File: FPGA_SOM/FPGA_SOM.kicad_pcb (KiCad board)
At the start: 6 copper layers, 42 x 38 mm, 47 parts, among them J102 Conn_01x14, J103 Conn_01x09, J104 Conn_01x11, J105 Conn_01x02, J106 Conn_01x06, U102 AP2127N-3.3, U103 W25X20CLSN, U104 AP2127N-1.2, U105 ICE40UP5K-SG48ITR, X101 ECS-2520MV-xxx-xx

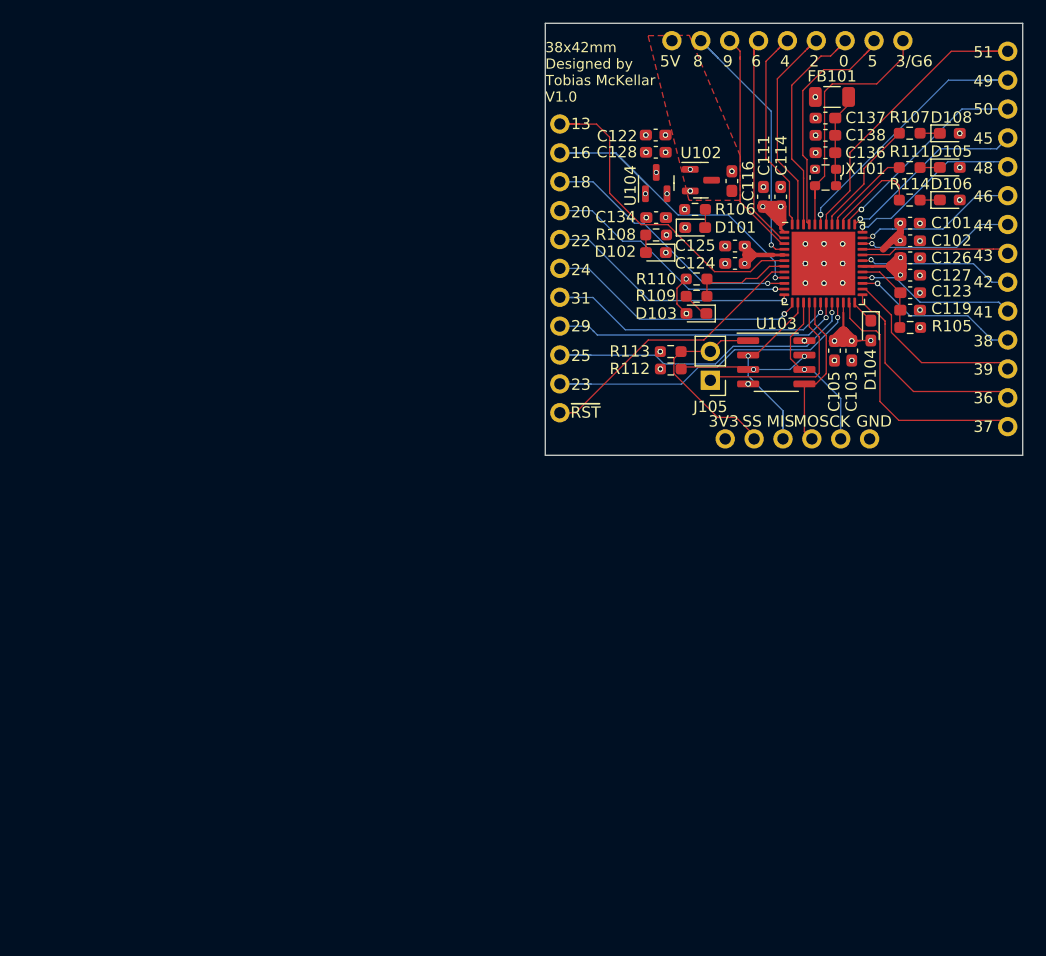
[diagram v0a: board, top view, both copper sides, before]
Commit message: First attempt at V2. Likely to be changed in the near future.
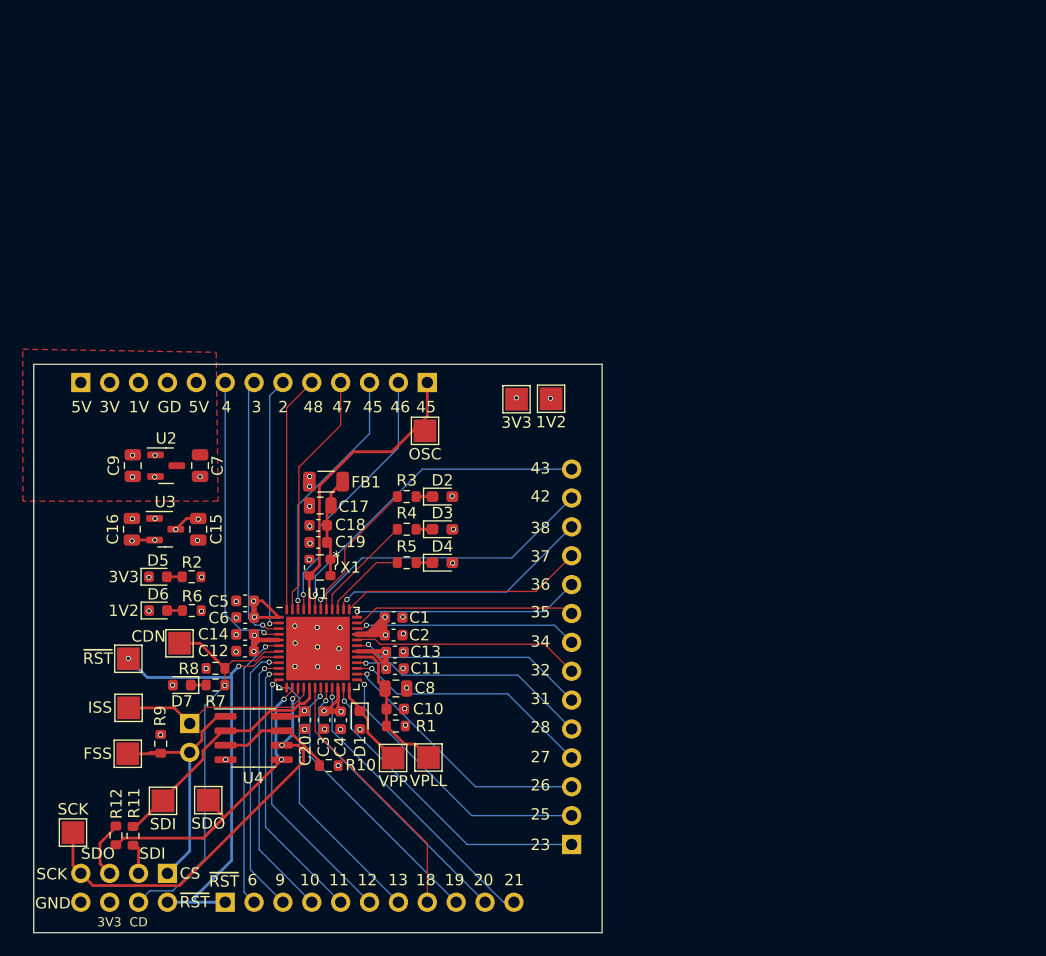
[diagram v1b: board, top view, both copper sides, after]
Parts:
- removed C101, C103, C111, C123, C124, C125, C138: 100n, Capacitor_SMD:C_0603_1608Metric_Pad1.08x0.95mm_HandSolder
- removed C102, C105, C114, C126, C127, C136: 10n, Capacitor_SMD:C_0603_1608Metric_Pad1.08x0.95mm_HandSolder
- removed C116, C119, C122, C128, C137: 10u, Capacitor_SMD:C_0603_1608Metric_Pad1.08x0.95mm_HandSolder
- removed C134: 22u, Capacitor_SMD:C_0603_1608Metric_Pad1.08x0.95mm_HandSolder
- removed D101, D102, D103: LED, Diode_SMD:D_0603_1608Metric_Pad1.05x0.95mm_HandSolder
- removed D104: 1N4004, Diode_SMD:D_0603_1608Metric_Pad1.05x0.95mm_HandSolder
- removed D105, D106, D108: LED_Small, Diode_SMD:D_0603_1608Metric_Pad1.05x0.95mm_HandSolder
- removed FB101: FerriteBead, Resistor_SMD:R_1206_3216Metric
- removed J102: Conn_01x14, Connector_PinHeader_2.54mm:PinHeader_1x14_P2.54mm_Vertical
- removed J103: Conn_01x09, Connector_PinHeader_2.54mm:PinHeader_1x09_P2.54mm_Vertical
- removed J104: Conn_01x11, Connector_PinHeader_2.54mm:PinHeader_1x11_P2.54mm_Vertical
- removed J105: Conn_01x02, Connector_PinHeader_2.54mm:PinHeader_1x02_P2.54mm_Vertical
- removed J106: Conn_01x06, Connector_PinHeader_2.54mm:PinHeader_1x06_P2.54mm_Vertical
- removed R105: 100, Resistor_SMD:R_0603_1608Metric_Pad0.98x0.95mm_HandSolder
- removed R106, R109: 2k2, Resistor_SMD:R_0603_1608Metric_Pad0.98x0.95mm_HandSolder
- removed R107, R108, R111, R114: 1k, Resistor_SMD:R_0603_1608Metric_Pad0.98x0.95mm_HandSolder
- removed R110: 5k, Resistor_SMD:R_0603_1608Metric_Pad0.98x0.95mm_HandSolder
- removed R112, R113: 10k, Resistor_SMD:R_0603_1608Metric_Pad0.98x0.95mm_HandSolder
- removed U102: AP2127N-3.3, Package_TO_SOT_SMD:SOT-23
- removed U103: W25X20CLSN, Package_SO:SOIC-8_3.9x4.9mm_P1.27mm
- removed U104: AP2127N-1.2, Package_TO_SOT_SMD:SOT-23
- removed U105: ICE40UP5K-SG48ITR, Package_DFN_QFN:QFN-48-1EP_7x7mm_P0.5mm_EP5.6x5.6mm
- removed X101: ECS-2520MV-xxx-xx, Oscillator:Oscillator_SMD_ECS_2520MV-xxx-xx-4Pin_2.5x2.0mm
- added ?: VPP, TestPoint:TestPoint_Pad_2.0x2.0mm, F.Cu at (131.6, 134.6)
- added C1: 100n, Capacitor_SMD:C_0603_1608Metric, F.Cu at (131.7, 122.3)
- added C10: 100n, Capacitor_SMD:C_0603_1608Metric, F.Cu at (131.8, 130.3)
- added C11: 100n, Capacitor_SMD:C_0603_1608Metric, F.Cu at (131.8, 126.8)
- added C12: 100n, Capacitor_SMD:C_0603_1608Metric, F.Cu at (118.6, 125.2)
- added C13: 10n, Capacitor_SMD:C_0603_1608Metric, F.Cu at (131.8, 125.3)
- added C14: 10n, Capacitor_SMD:C_0603_1608Metric, F.Cu at (118.6, 123.8)
- added C15: 10u, Capacitor_SMD:C_0805_2012Metric, F.Cu at (114.5, 114.5)
- added C16: 22u, Capacitor_SMD:C_0805_2012Metric, F.Cu at (108.6, 114.5)
- added C17: 10u, Capacitor_SMD:C_0805_2012Metric, F.Cu at (125.2, 112.4)
- added C18: 100n, Capacitor_SMD:C_0603_1608Metric, F.Cu at (125.0, 114.2)
- added C19: 10n, Capacitor_SMD:C_0603_1608Metric, F.Cu at (125.0, 115.7)
- added C2: 10n, Capacitor_SMD:C_0603_1608Metric, F.Cu at (131.7, 123.8)
- added C20: 100n, Capacitor_SMD:C_0603_1608Metric, F.Cu at (123.8, 131.3)
- added C3: 100n, Capacitor_SMD:C_0603_1608Metric, F.Cu at (125.5, 131.3)
- added C4: 10n, Capacitor_SMD:C_0603_1608Metric, F.Cu at (127.0, 131.3)
- added C5: 100n, Capacitor_SMD:C_0603_1608Metric, F.Cu at (118.6, 120.8)
- added C6: 10n, Capacitor_SMD:C_0603_1608Metric, F.Cu at (118.6, 122.3)
- added C7: 10u, Capacitor_SMD:C_0805_2012Metric, F.Cu at (114.6, 108.9)
- added C8: 10u, Capacitor_SMD:C_0805_2012Metric, F.Cu at (131.9, 128.5)
- added C9: 10u, Capacitor_SMD:C_0805_2012Metric, F.Cu at (108.7, 108.9)
- added D1: 1N4004, Diode_SMD:D_0603_1608Metric, F.Cu at (128.7, 131.3)
- added D2: LED_Small, Diode_SMD:D_0603_1608Metric_Pad1.05x0.95mm_HandSolder, F.Cu at (135.9, 111.6)
- added D3: LED_Small, Diode_SMD:D_0603_1608Metric_Pad1.05x0.95mm_HandSolder, F.Cu at (135.9, 114.5)
- added D4: LED_Small, Diode_SMD:D_0603_1608Metric_Pad1.05x0.95mm_HandSolder, F.Cu at (135.9, 117.5)
- added D5: LED, Diode_SMD:D_0603_1608Metric, F.Cu at (110.9, 118.7)
- added D6: LED, Diode_SMD:D_0603_1608Metric, F.Cu at (110.9, 121.7)
- added D7: LED, Diode_SMD:D_0603_1608Metric, F.Cu at (113.0, 128.2)
- added FB1: FerriteBead, Resistor_SMD:R_1206_3216Metric, F.Cu at (125.7, 110.3)
- added J1: Conn_01x14, Connector_PinHeader_2.54mm:PinHeader_1x14_P2.54mm_Vertical, F.Cu at (147.3, 142.2)
- added J2: Conn_01x09, Connector_PinHeader_2.54mm:PinHeader_1x09_P2.54mm_Vertical, F.Cu at (134.6, 101.6)
- added J3: Conn_01x11, Connector_PinHeader_2.54mm:PinHeader_1x11_P2.54mm_Vertical, F.Cu at (116.8, 147.3)
- added J4: Conn_01x04, Connector_PinHeader_2.54mm:PinHeader_1x04_P2.54mm_Vertical, F.Cu at (104.1, 101.6)
- added J5: Conn_01x02, Connector_PinHeader_2.54mm:PinHeader_1x02_P2.54mm_Vertical, F.Cu at (113.7, 131.6)
- added J6: Conn_02x04_Counter_Clockwise, Connector_PinHeader_2.54mm:PinHeader_2x04_P2.54mm_Vertical, F.Cu at (111.8, 144.8)
- added R1: 100, Resistor_SMD:R_0603_1608Metric, F.Cu at (131.9, 131.8)
- added R10: 10k, Resistor_SMD:R_0603_1608Metric, F.Cu at (126.0, 135.3)
- added R11: 0, Resistor_SMD:R_0603_1608Metric, F.Cu at (108.7, 141.5)
- added R12: 0, Resistor_SMD:R_0603_1608Metric, F.Cu at (107.2, 141.4)
- added R2: 2k2, Resistor_SMD:R_0603_1608Metric, F.Cu at (113.9, 118.7)
- added R3: 1k, Resistor_SMD:R_0603_1608Metric, F.Cu at (132.8, 111.6)
- added R4: 1k, Resistor_SMD:R_0603_1608Metric, F.Cu at (132.8, 114.5)
- added R5: 1k, Resistor_SMD:R_0603_1608Metric, F.Cu at (132.8, 117.5)
- added R6: 1k, Resistor_SMD:R_0603_1608Metric, F.Cu at (113.9, 121.7)
- added R7: 2k2, Resistor_SMD:R_0603_1608Metric, F.Cu at (116.0, 128.2)
- added R8: 4k7, Resistor_SMD:R_0603_1608Metric, F.Cu at (116.0, 126.7)
- added R9: 10k, Resistor_SMD:R_0603_1608Metric, F.Cu at (111.2, 133.4)
- added TP10: ~{RST}, TestPoint:TestPoint_Pad_2.0x2.0mm, F.Cu at (108.3, 125.9)
- added TP11: CDN, TestPoint:TestPoint_Pad_2.0x2.0mm, F.Cu at (112.8, 124.5)
- added TP12: OSC, TestPoint:TestPoint_Pad_2.0x2.0mm, F.Cu at (134.4, 105.8)
- added TP2: VPLL, TestPoint:TestPoint_Pad_2.0x2.0mm, F.Cu at (134.7, 134.6)
- added TP3: 3V3, TestPoint:TestPoint_Pad_2.0x2.0mm, F.Cu at (142.5, 103.1)
- added TP4: 1V2, TestPoint:TestPoint_Pad_2.0x2.0mm, F.Cu at (145.5, 103.0)
- added TP5: FSS, TestPoint:TestPoint_Pad_2.0x2.0mm, F.Cu at (108.3, 134.3)
- added TP6: ISS, TestPoint:TestPoint_Pad_2.0x2.0mm, F.Cu at (108.3, 130.2)
- added TP7: SCK, TestPoint:TestPoint_Pad_2.0x2.0mm, F.Cu at (103.5, 141.2)
- added TP8: SDO, TestPoint:TestPoint_Pad_2.0x2.0mm, F.Cu at (115.3, 138.3)
- added TP9: SDI, TestPoint:TestPoint_Pad_2.0x2.0mm, F.Cu at (111.4, 138.4)
- added U1: ICE40UP5K-SG48ITR, Package_DFN_QFN:QFN-48-1EP_7x7mm_P0.5mm_EP5.6x5.6mm, F.Cu at (125.0, 125.0)
- added U2: AP2127N-3.3, Package_TO_SOT_SMD:SOT-23, F.Cu at (111.6, 108.9)
- added U3: AP2127N-1.2, Package_TO_SOT_SMD:SOT-23, F.Cu at (111.6, 114.5)
- added U4: W25X20CLSN, Package_SO:SOIC-8_3.9x4.9mm_P1.27mm, F.Cu at (119.3, 132.9)
- added X1: ECS-2520MV-xxx-xx, Oscillator:Oscillator_SMD_ECS_2520MV-xxx-xx-4Pin_2.5x2.0mm, F.Cu at (125.2, 117.9)
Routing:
- net Net-(J104-Pin_2): track 33.0 -> 0.00 mm, vias 1 -> 0
- net Net-(J104-Pin_10): track 31.2 -> 0.00 mm, vias 1 -> 0
- net Net-(J104-Pin_1): track 30.0 -> 0.00 mm
- net Net-(J104-Pin_9): track 29.9 -> 0.00 mm, vias 1 -> 0
- net Net-(J1-Pin_14): track 0.00 -> 29.4 mm, vias 0 -> 1
- net Net-(J1-Pin_1): track 0.00 -> 27.5 mm, vias 0 -> 1
- net Net-(J1-Pin_13): track 0.00 -> 26.7 mm, vias 0 -> 1
- net Net-(J104-Pin_7): track 26.6 -> 0.00 mm, vias 1 -> 0
- net Net-(J102-Pin_14): track 26.2 -> 0.00 mm
- net Net-(J3-Pin_11): track 0.00 -> 26.0 mm, vias 0 -> 1
- net Net-(J2-Pin_8): track 0.00 -> 25.8 mm, vias 0 -> 1
- net Net-(J104-Pin_8): track 25.8 -> 0.00 mm, vias 1 -> 0
- net /CDONE: track 9.61 -> 35.2 mm, vias 0 -> 1
- net Net-(J3-Pin_10): track 0.00 -> 25.3 mm, vias 0 -> 1
- net Net-(J1-Pin_2): track 0.00 -> 25.1 mm, vias 0 -> 1
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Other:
- board size 42 x 38 mm -> 50 x 50 mm
- board text added: "*"
- board text added: "10"
- board text added: "11"
- board text added: "12"
- board text added: "19"
- board text added: "1V"
- board text added: "1V2"
- board text added: "21"
- board text added: "26"
- board text added: "27"
- board text added: "28"
- board text added: "3"
- board text added: "32"
- board text added: "34"
- board text added: "35"
- board text added: "3V"
- board text added: "47"
- board text added: "CD"
- board text added: "CS"
- board text added: "GD"
- board text added: "SCK"
- board text added: "SDI"
- board text added: "SDO"
- board text removed: "0"
- board text removed: "16"
- board text removed: "22"
- board text removed: "24"
- board text removed: "29"
- board text removed: "3/G6"
- board text removed: "38x42mm Designed by Tobias McKellar V1.0"
- board text removed: "39"
- board text removed: "41"
- board text removed: "44"
- board text removed: "49"
- board text removed: "5"
- board text removed: "50"
- board text removed: "51"
- board text removed: "8"
- board text removed: "CK"
- board text removed: "JLCJLCJLCJLC"
- board text removed: "MIS"
- board text removed: "MOS"
- board text removed: "SS"
